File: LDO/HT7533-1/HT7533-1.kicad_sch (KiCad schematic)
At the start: 5 parts

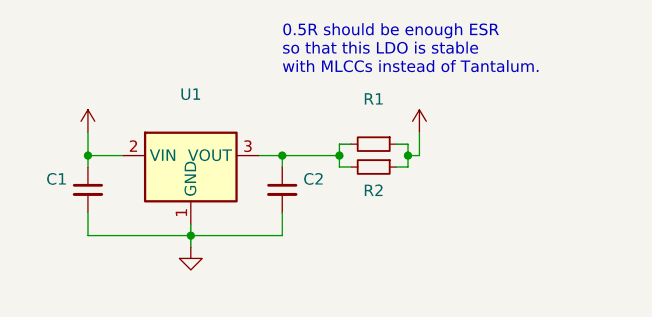
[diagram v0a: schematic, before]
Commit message: Reapply "Update modules to kicad v7 format"
This reverts commit fa5cc85431189ac7a3beedf0871b5723203ae43f.
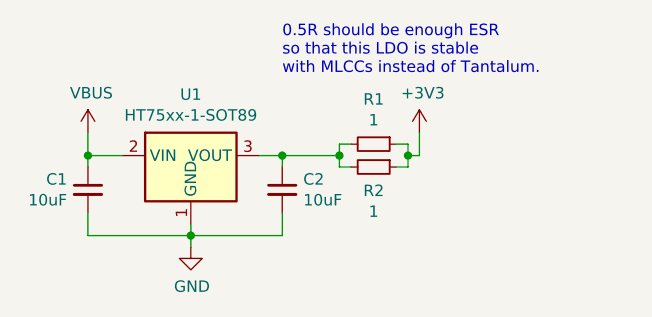
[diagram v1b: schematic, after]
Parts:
- C1, C2: value (none) -> 10uF; footprint (none) -> Capacitor_SMD:C_0603_1608Metric
- R1, R2: value (none) -> 1; footprint (none) -> Resistor_SMD:R_0402_1005Metric
- U1: value (none) -> HT75xx-1-SOT89; footprint (none) -> Package_TO_SOT_SMD:SOT-89-3
